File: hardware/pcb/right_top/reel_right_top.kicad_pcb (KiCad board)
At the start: 2 copper layers, 145 x 88.1 mm, 23 parts, among them SW1 choc_plate, SW10 choc_plate, SW11 choc_plate, SW12 choc_plate, SW13 choc_plate, SW14 choc_plate, SW15 choc_plate, SW16 choc_plate, SW17 choc_plate, SW18 choc_plate, SW19 choc_plate, SW2 choc_plate, SW3 choc_plate, SW4 choc_plate, SW5 choc_plate, SW6 choc_plate, SW7 choc_plate, SW8 choc_plate, SW9 choc_plate

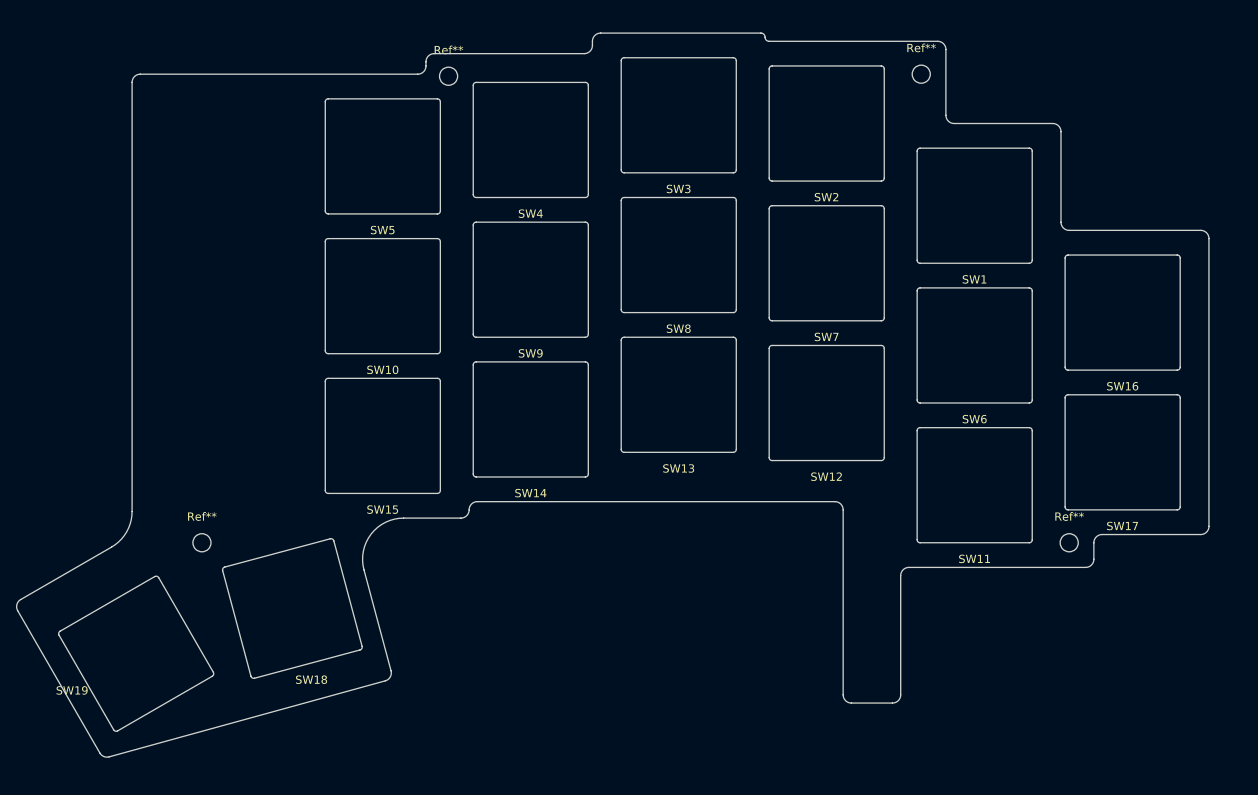
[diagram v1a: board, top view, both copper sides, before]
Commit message: Publish current hardware and fabrication assets
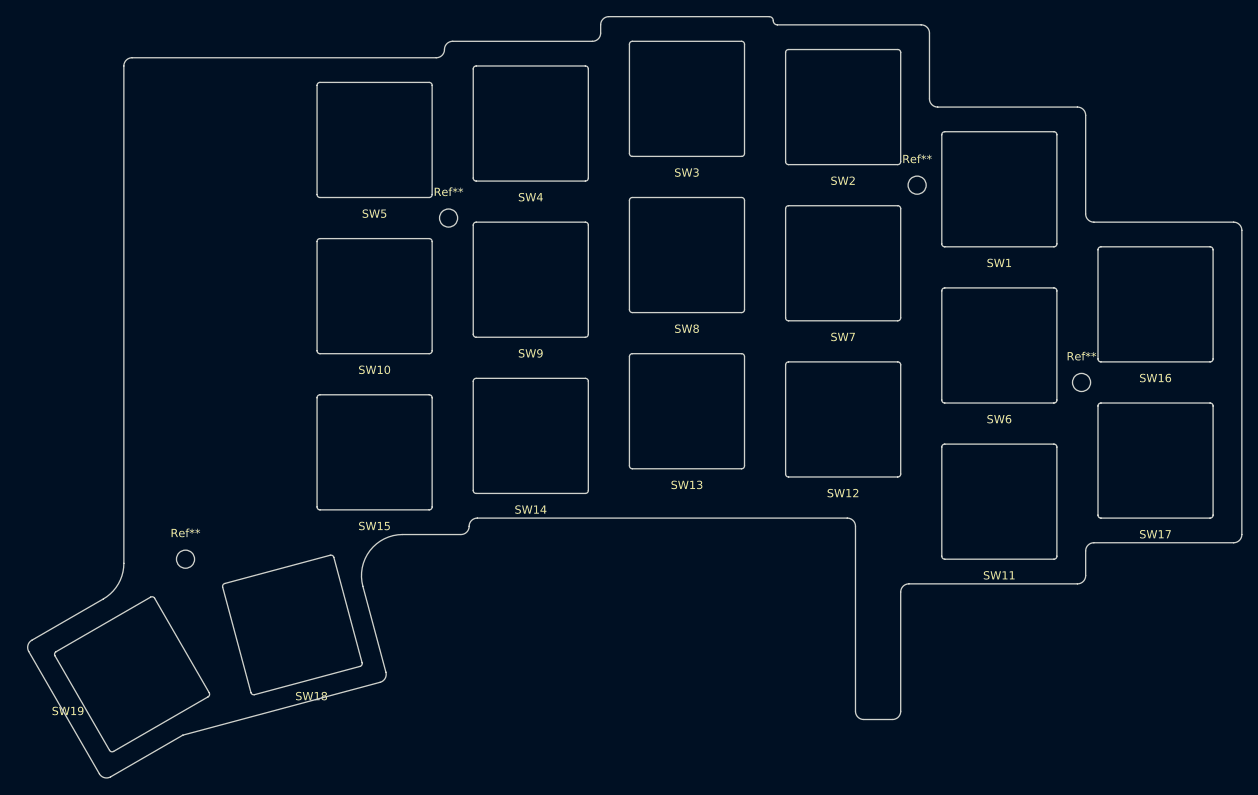
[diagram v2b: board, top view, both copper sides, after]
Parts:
- removed the Ref** at (163.5, 107.5)
- removed the Ref** at (145.5, 50.5)
- removed the Ref** at (58.0, 107.5)
- removed the Ref** at (88.0, 50.8)
- added Ref**: MountingHole_2.2mm_M2, MountingHole:MountingHole_2.2mm_M2, F.Cu at (56.0, 109.5)
- added Ref**: MountingHole_2.2mm_M2, MountingHole:MountingHole_2.2mm_M2, F.Cu at (88.0, 68.0)
- added Ref**: MountingHole_2.2mm_M2, MountingHole:MountingHole_2.2mm_M2, F.Cu at (165.0, 88.0)
- added Ref**: MountingHole_2.2mm_M2, MountingHole:MountingHole_2.2mm_M2, F.Cu at (145.0, 64.0)
- moved SW16 4.12 mm to (174.0, 78.5)
- moved SW17 4.12 mm to (174.0, 97.5)
- moved SW1 3.61 mm to (155.0, 64.5)
- moved SW11 3.61 mm to (155.0, 102.5)
- moved SW6 3.00 mm to (155.0, 83.5)
- moved SW12 2.83 mm to (136.0, 92.5)
- moved SW2 2.83 mm to (136.0, 54.5)
- moved SW19 2.55 mm to (49.5, 123.5)
- moved SW13 2.24 mm to (117.0, 91.5)
- moved SW15 2.24 mm to (79.0, 96.5)
- moved SW3 2.24 mm to (117.0, 53.5)
- moved SW5 2.24 mm to (79.0, 58.5)
- moved SW14 2.00 mm to (98.0, 94.5)
- moved SW18 2.00 mm to (69.0, 117.5)
- moved SW4 2.00 mm to (98.0, 56.5)
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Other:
- board size 145 x 88.1 mm -> 147.7 x 92.6 mm
